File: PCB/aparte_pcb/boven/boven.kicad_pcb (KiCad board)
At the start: 2 copper layers, 100.5 x 100.5 mm, 51 parts, among them IC1 TSSP4038, IC10 TSSP4038, IC11 TSSP4038, IC12 TSSP4038, IC13 TSSP4038, IC14 TSSP4038, IC15 TSSP4038, IC16 TSSP4038, IC2 TSSP4038, IC3 TSSP4038, IC4 TSSP4038, IC5 TSSP4038, IC6 TSSP4038, IC7 TSSP4038, IC8 TSSP4038, IC9 TSSP4038, J1 Conn_01x10_Socket, J2 Screw_Terminal_01x01, J3 Screw_Terminal_01x01, J4 Screw_Terminal_01x01, SW1 SW_DPST_x2, U1 openMV_M7_R2

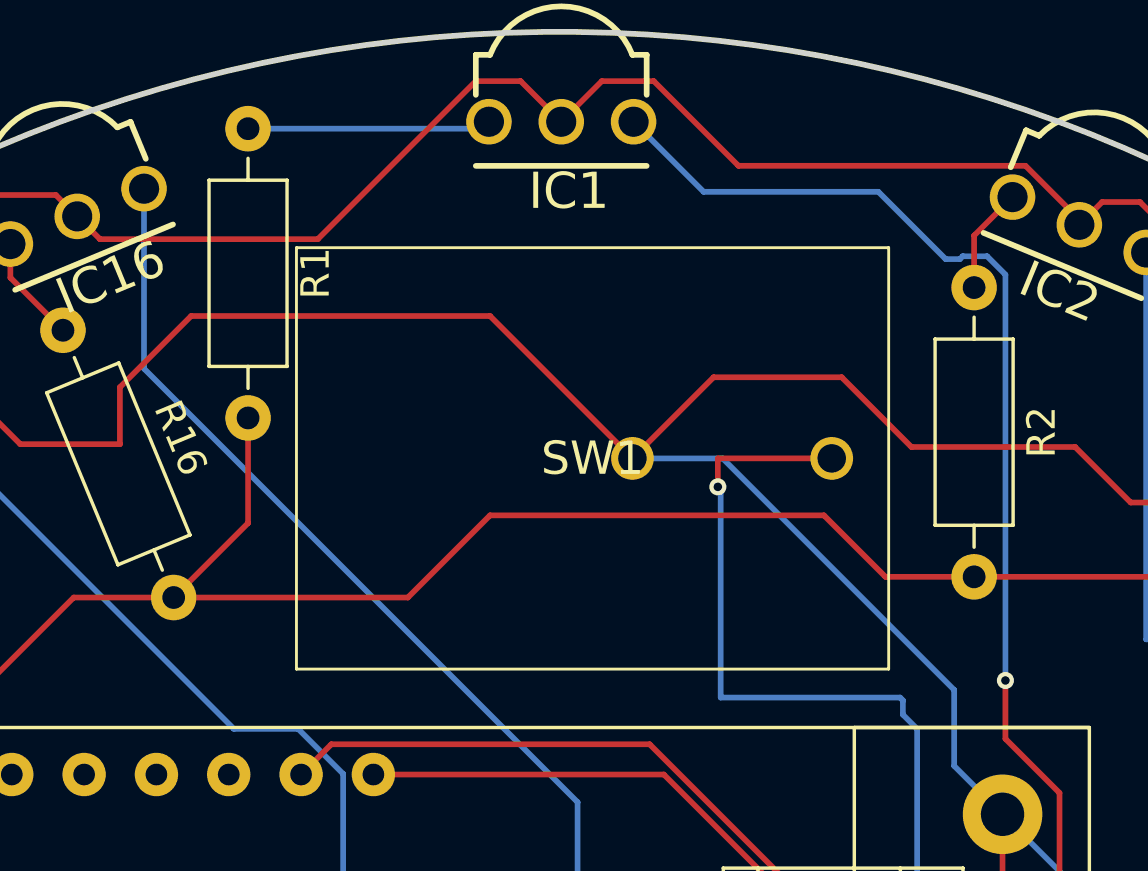
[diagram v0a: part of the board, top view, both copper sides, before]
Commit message: dgsrf
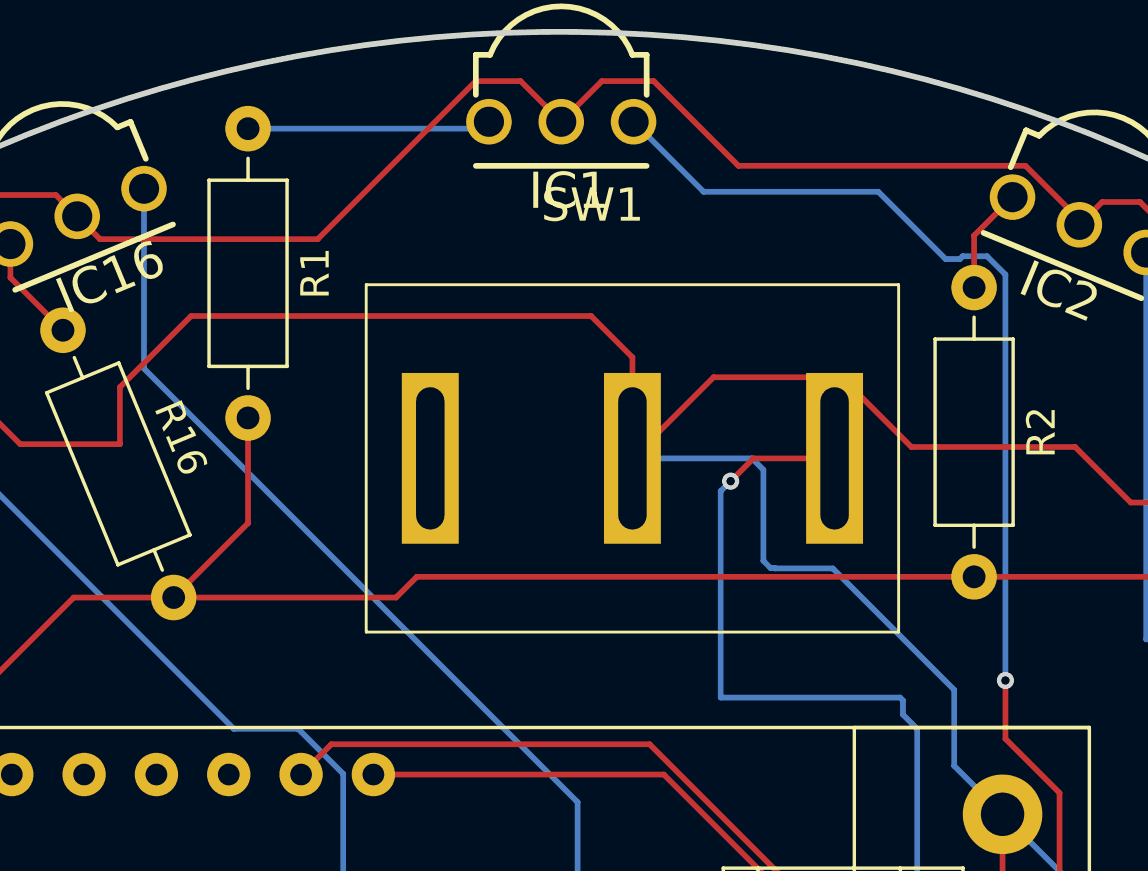
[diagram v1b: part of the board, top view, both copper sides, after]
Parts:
- SW1: footprint Library:R1966ABLKBLKEF -> Library:Rocker Switch 3-Pin, SPDT, 10A
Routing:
- net Net-(D11-A): track 296.3 -> 300.3 mm
- net Net-(D1-K): track 268.2 -> 266.4 mm
- net soft_power_sw: track 27.6 -> 26.8 mm
